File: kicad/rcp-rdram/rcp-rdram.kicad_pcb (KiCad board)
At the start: 2 copper layers, 47.1 x 49.7 mm, 32 parts, among them P1 RDRAM-EDGE, U11 RDRAM18-NUS, U11-2 RDRAM18-NUS, U14 RDRAM18-NUS, U14-2 RDRAM18-NUS, U15 MX8330, X2 14.705MHz

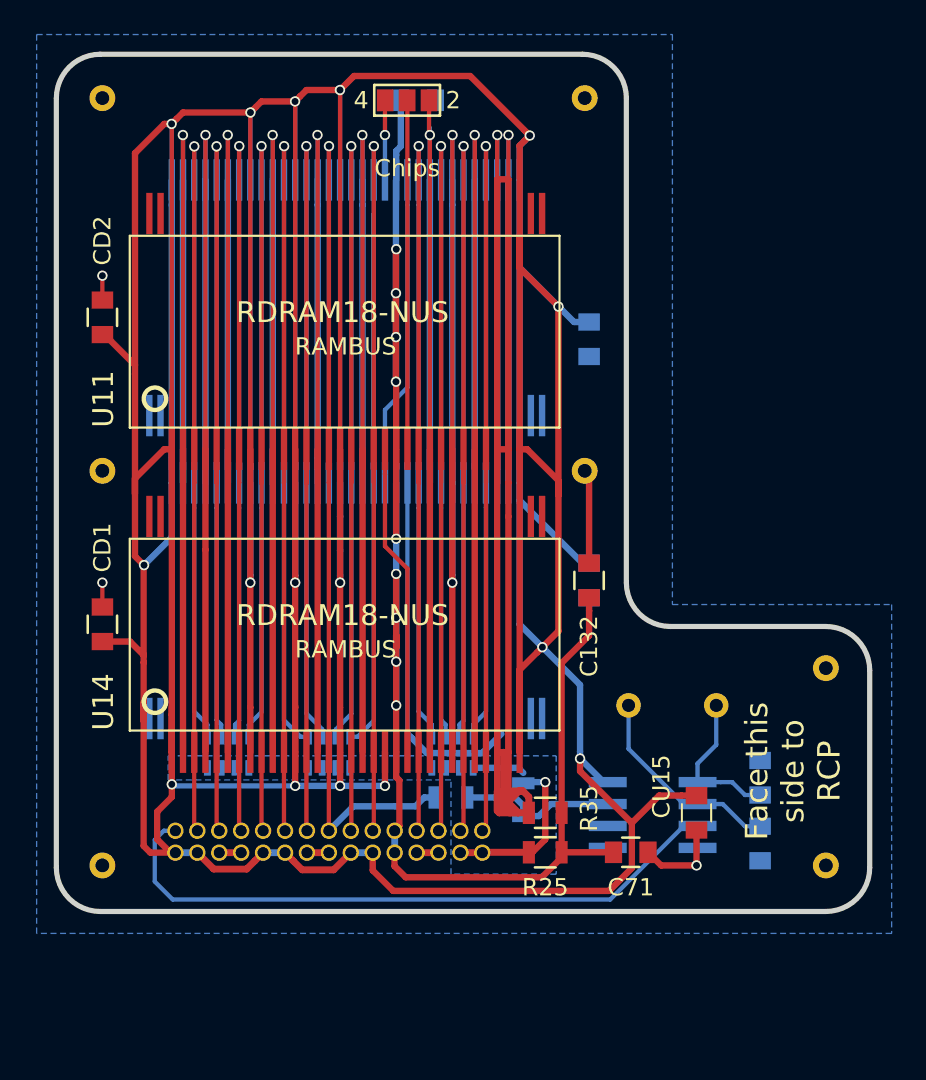
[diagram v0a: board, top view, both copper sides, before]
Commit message: Minor cleanups
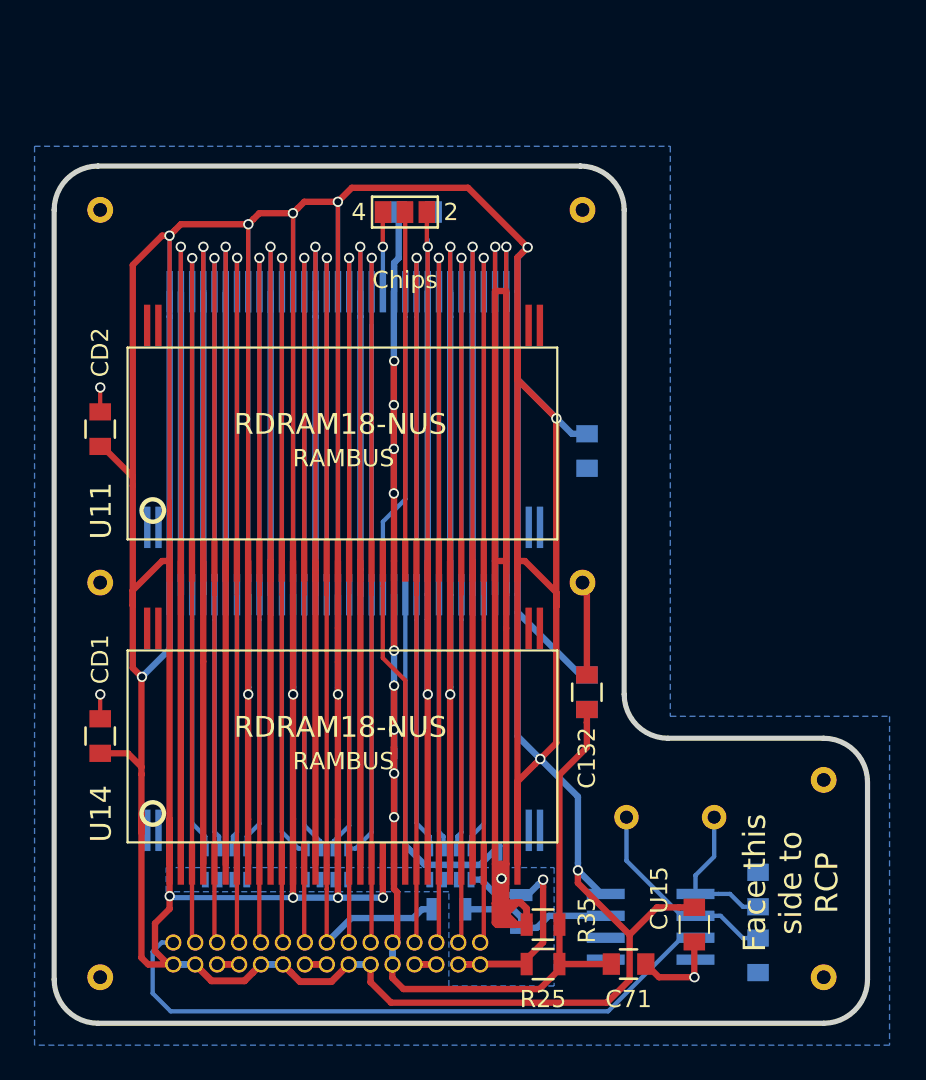
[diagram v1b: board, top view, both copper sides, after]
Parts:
- moved C71 6.48 mm to (56.0, 70.5)
- moved R25 6.48 mm to (51.1, 70.5)
- moved REF** 6.48 mm to (67.3, 71.2)
- moved REF** 6.48 mm to (25.4, 71.2)
- moved C132 6.48 mm to (53.6, 54.7)
- moved CD1 6.48 mm to (25.4, 57.3)
- moved CU15 6.48 mm to (59.8, 68.2)
- moved JP1 6.48 mm to (43.1, 26.9)
- moved R35 6.48 mm to (51.1, 68.2)
- moved REF** 6.48 mm to (25.4, 26.8)
- moved REF** 6.48 mm to (25.4, 48.4)
- moved REF** 6.48 mm to (53.3, 26.8)
- moved REF** 6.48 mm to (53.3, 48.4)
- moved U11 6.48 mm to (39.5, 41.2)
- moved U14 6.48 mm to (39.5, 58.7)
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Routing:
- net GND: track 685.7 -> 695.0 mm, vias 15 -> 17
- net /VTERM: track 12.9 -> 14.2 mm
